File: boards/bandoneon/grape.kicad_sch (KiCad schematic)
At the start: 9 parts, among them U3 MCP3008

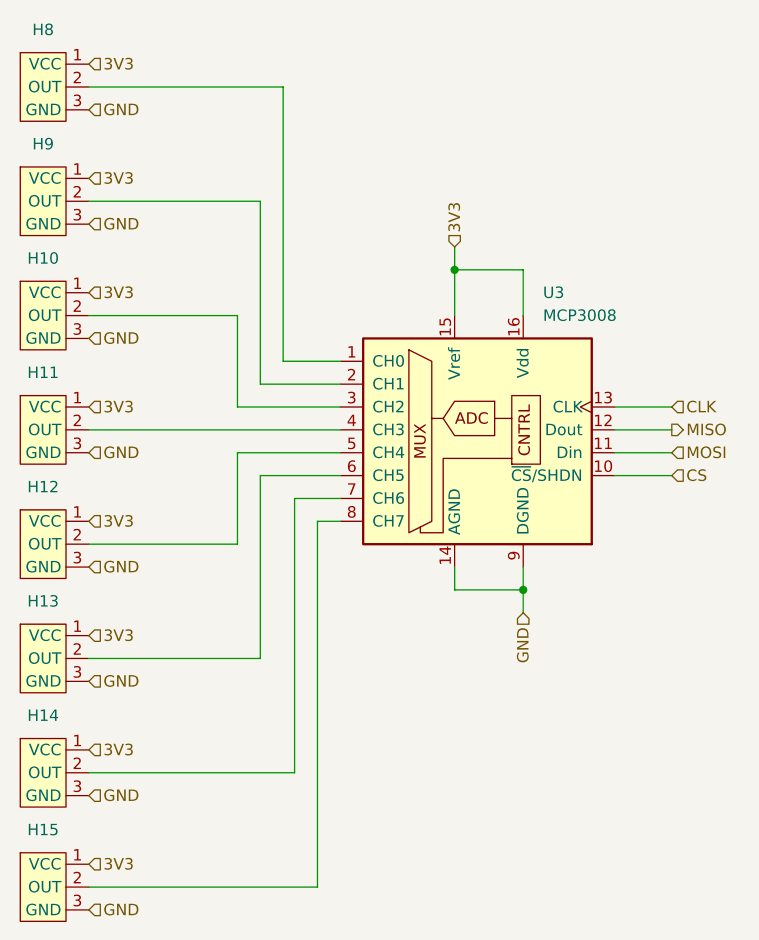
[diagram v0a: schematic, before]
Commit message: Ready for routing
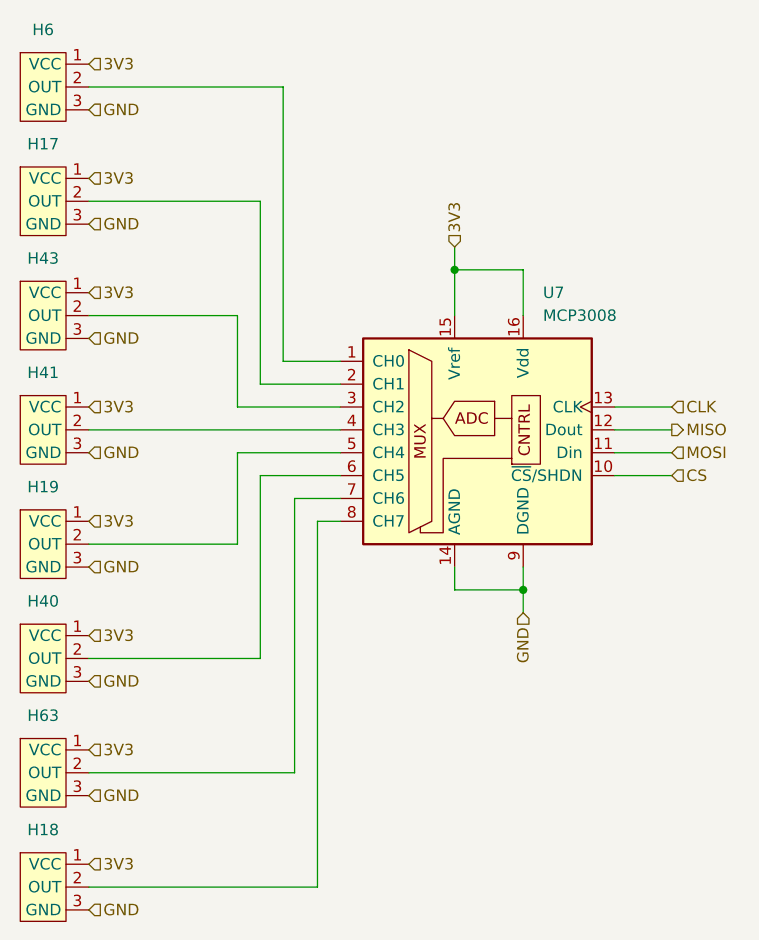
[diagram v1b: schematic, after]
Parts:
- renumbered H9 to H17, H15 to H18, H12 to H19, H13 to H40, H11 to H41, H10 to H43, H8 to H6, H14 to H63, U3 to U7

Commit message: Manual routing
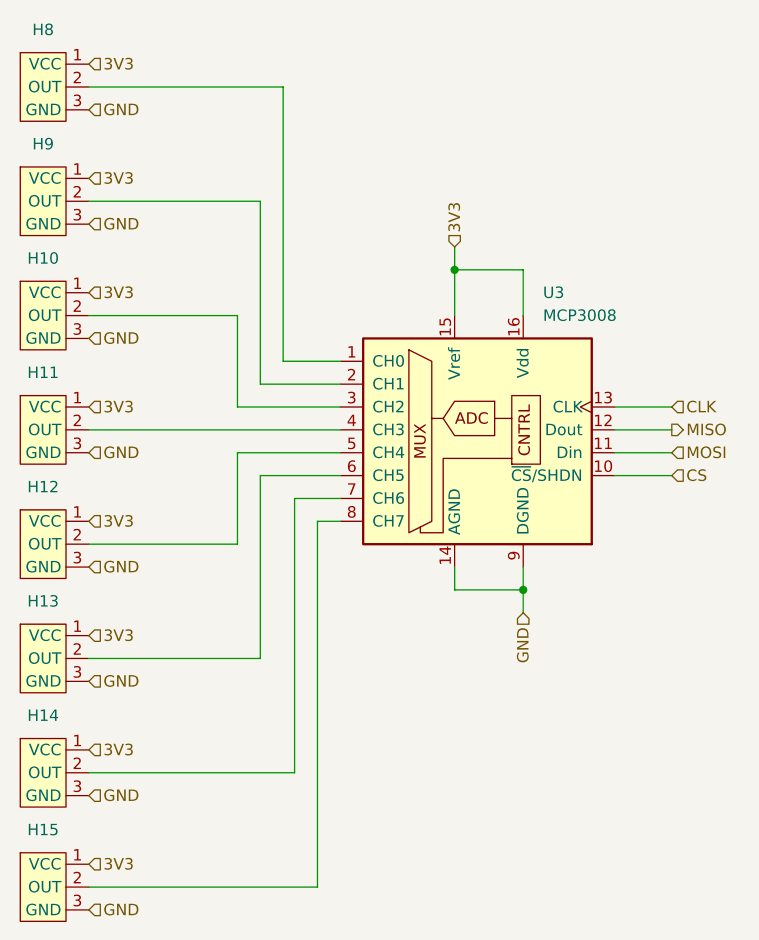
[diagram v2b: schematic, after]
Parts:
- renumbered H43 to H10, H41 to H11, H19 to H12, H40 to H13, H63 to H14, H18 to H15, H6 to H8, H17 to H9, U7 to U3
